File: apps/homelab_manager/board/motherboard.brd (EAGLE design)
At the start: 74.6 x 55.9 mm, 59 parts

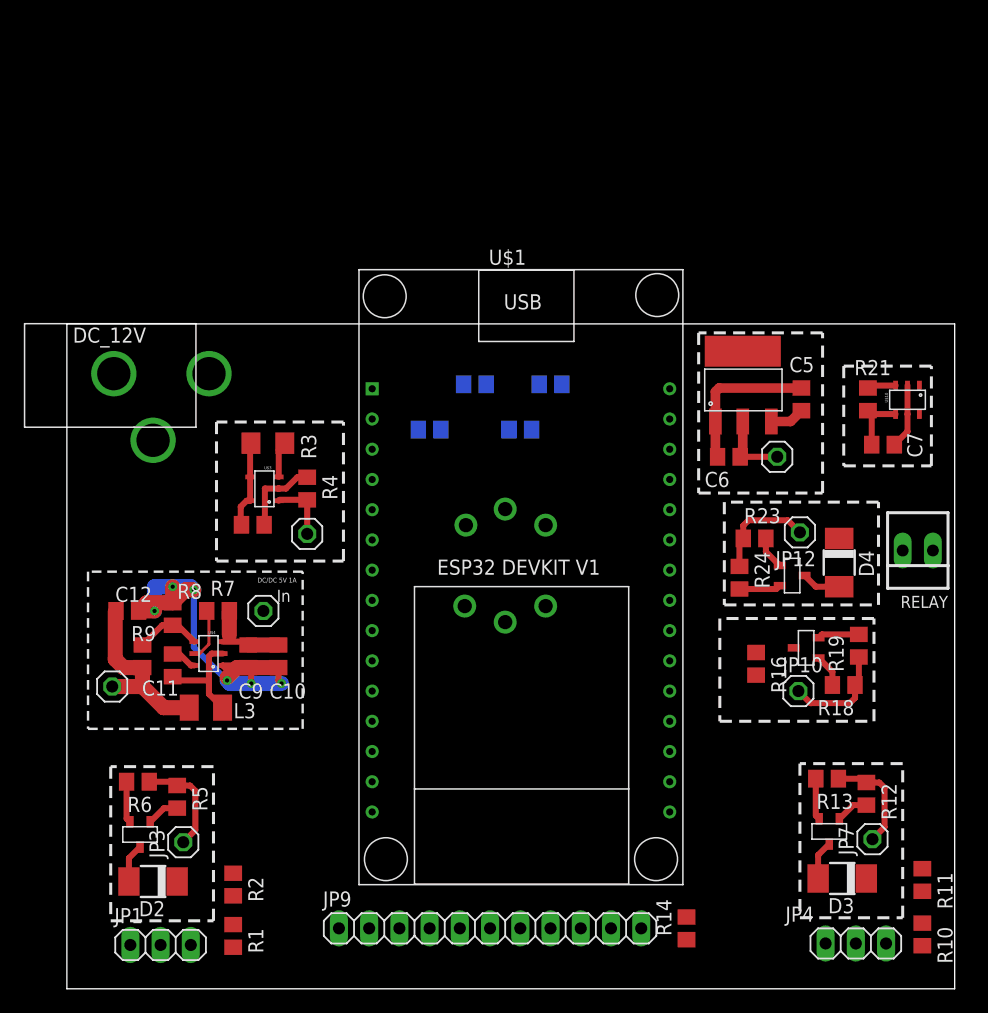
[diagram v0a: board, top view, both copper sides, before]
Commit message: motherboard (wip)
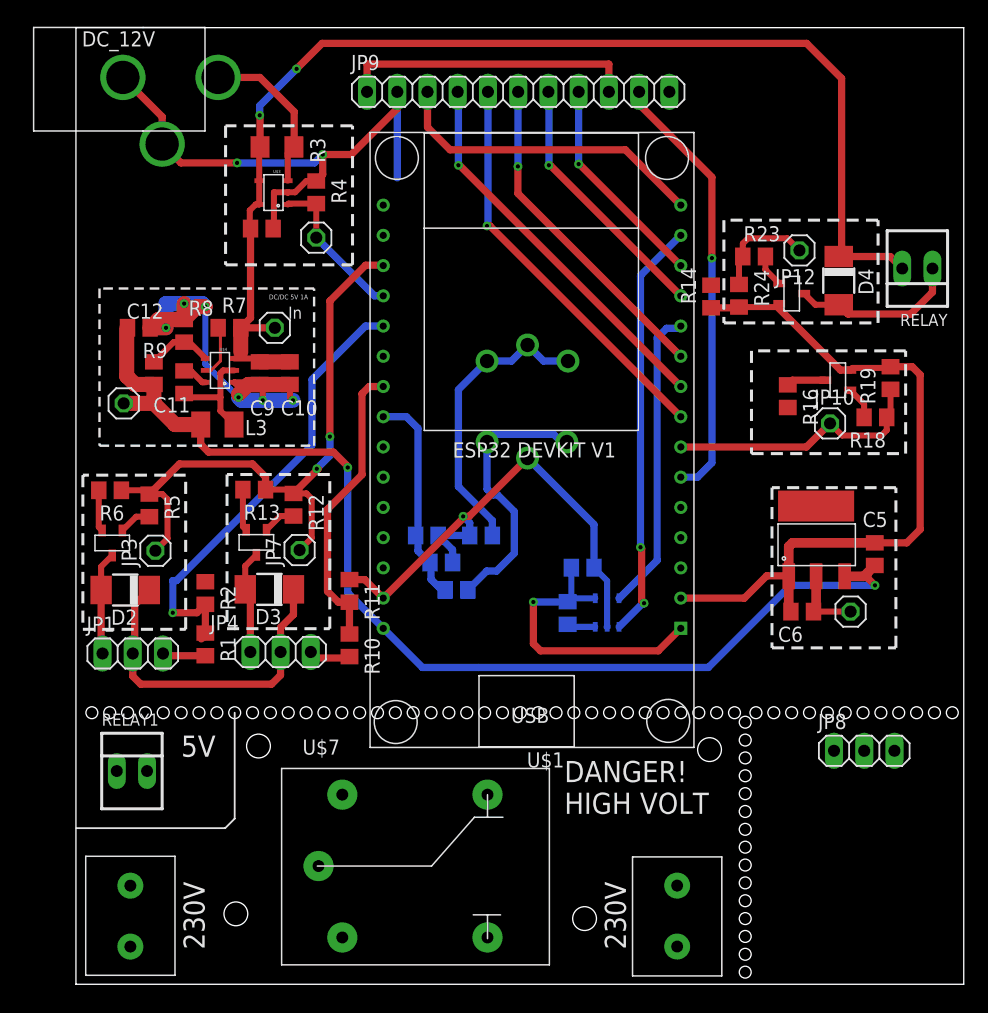
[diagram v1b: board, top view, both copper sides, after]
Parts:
- added JP8: SWITCH_LED, pinhead:1X03
- added RELAY1: 22-23-2021, con-molex:22-23-2021
- added U$12, U$13: SCREW_TERMINAL, bzd:SCREW_TERMINAL
- added U$7: RELAY_SONGLE, bzd:RELAY_SONGLE
- JP9: value (none) -> UI
- moved JP9 70.3 mm to (37.9, 75.4)
- moved JP4 54.2 mm to (18.0, 28.3)
- moved JP7 53.9 mm to (19.6, 36.9)
- moved R10 53.9 mm to (23.7, 28.9)
- moved R11 53.9 mm to (23.7, 33.4)
- moved R12 53.9 mm to (19.0, 40.7)
- moved R13 53.9 mm to (15.7, 41.9)
- moved U$6 53.9 mm to (14.5, 36.9)
- moved D3 53.9 mm to (17.0, 33.6)
- moved R14 53.1 mm to (54.1, 58.2)
- moved U$10 31.9 mm to (46.9, 30.8), flipped to the bottom, turned to 90 degrees
- moved R21 31.0 mm to (42.1, 31.6), flipped to the bottom, turned to 90 degrees
- moved C7 27.3 mm to (43.3, 35.4), flipped to the bottom, turned to 180 degrees
- moved C2 24.9 mm to (16.4, 63.9)
- moved DC_12V 24.9 mm to (-2.79, 76.6)
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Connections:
- removed net N$7: JP9.9
- new net N$15: RELAY1.1, U$7.COMMAND_V-
- new net N$16: U$12.P$2, U$13.P$1
- new net N$17: U$12.P$1, U$7.V-
- new net N$18: U$13.P$2, U$7.NO_V+
- new net N$6: RELAY1.2, U$7.COMMAND_V+
- net 3.3V: now also JP9.9
- net FAN2_SENSE: now also U$1.PIN_21; no longer U$1.PIN_18
- net HOMELAB_POWER: now also U$1.PIN_4; no longer U$1.PIN_21
- net LED: now also U$1.PIN_6; no longer U$1.PIN_26
- net VOUT_CURRENT: now also U$1.PIN_18; no longer U$1.PIN_4
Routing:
- net GND: track 77.5 -> 198.3 mm, vias 6 -> 9
- net VIN_REG: track 14.2 -> 130.7 mm, vias 0 -> 2
- net 7V: track 18.4 -> 94.9 mm, vias 0 -> 2
- net 3.3V: track 4.58 -> 49.4 mm, vias 0 -> 1
- net FAN1_SENSE: track 0.00 -> 38.5 mm, vias 0 -> 1
- net SWITCH: track 0.00 -> 36.8 mm, vias 0 -> 1
- net FAN_SWITCH: track 17.9 -> 53.5 mm, vias 0 -> 2
- net I2C_SCL: track 0.00 -> 35.4 mm, vias 0 -> 2
- net SPI_CS0: track 0.00 -> 34.2 mm, vias 0 -> 1
- net SPI_CLK: track 0.00 -> 32.6 mm, vias 0 -> 1
- net EINK_DC: track 0.00 -> 27.9 mm, vias 0 -> 1
- net SPI_MOSI: track 0.00 -> 27.0 mm
- net I2C_SDA: track 0.00 -> 25.6 mm
- net 5V: track 6.17 -> 30.9 mm
- net FAN2_SENSE: track 0.00 -> 24.7 mm
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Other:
- board size 74.6 x 55.9 mm -> 74.6 x 80.4 mm
- board text added: "230V"
- board text added: "5V"
- board text added: "DANGER! HIGH VOLT"
